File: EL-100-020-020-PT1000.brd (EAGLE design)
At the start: 54 x 29.5 mm, 53 parts, among them U1 OPA2188AIDGKR, U16 24AA256-I/SN, U2 OPA2188AIDGKR, U4 ADS1015IDGST, X1 944-12-08-00, X2 944-12-08-00, X3 9012-26

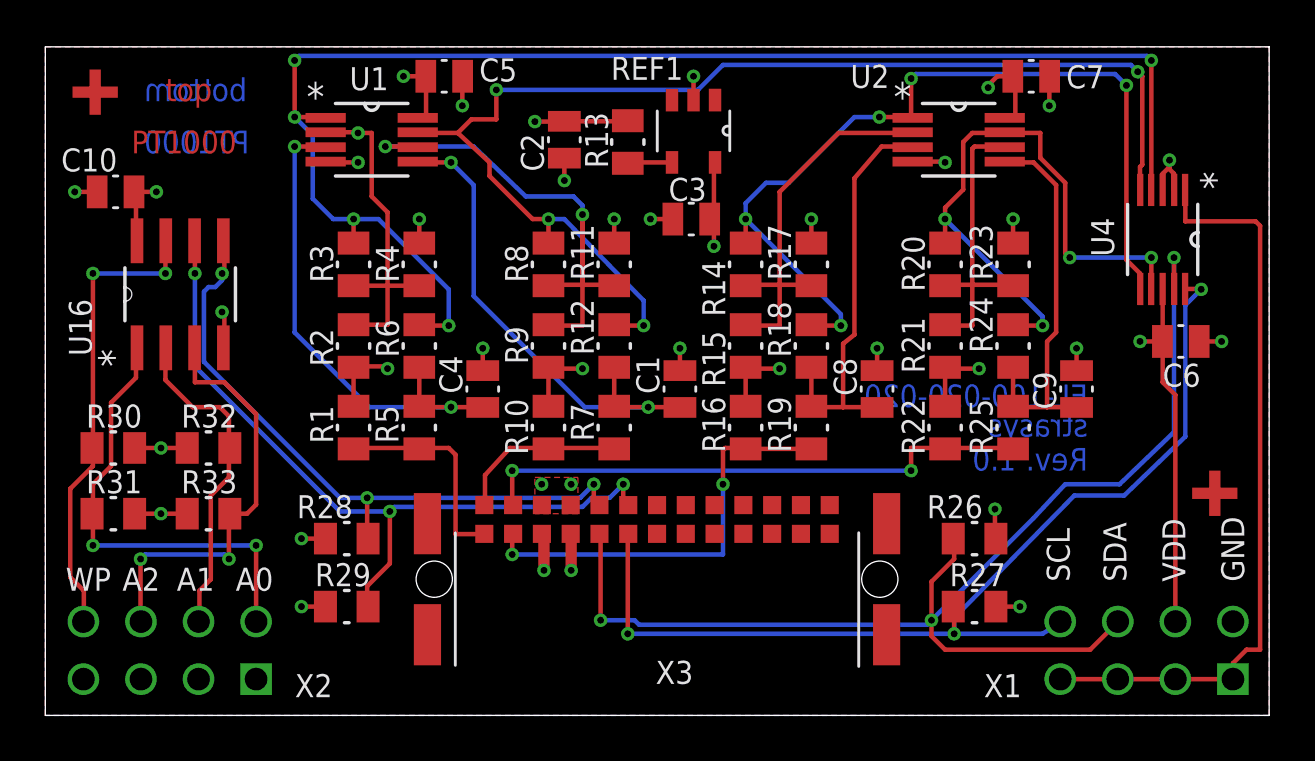
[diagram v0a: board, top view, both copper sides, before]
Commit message: DIN-Rail-production
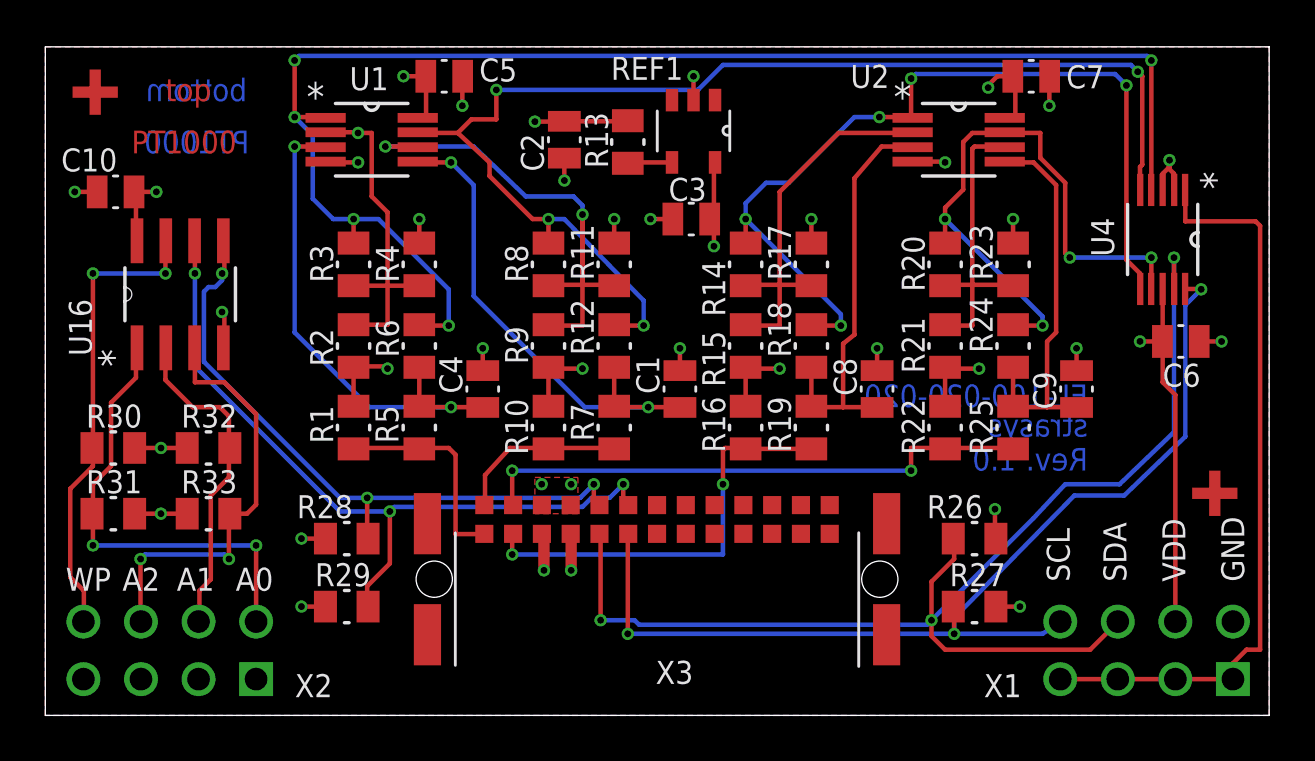
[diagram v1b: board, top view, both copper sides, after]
